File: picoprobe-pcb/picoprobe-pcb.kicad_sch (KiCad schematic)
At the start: 2 parts, among them J1 Conn_01x06_Pin, U1 Pico

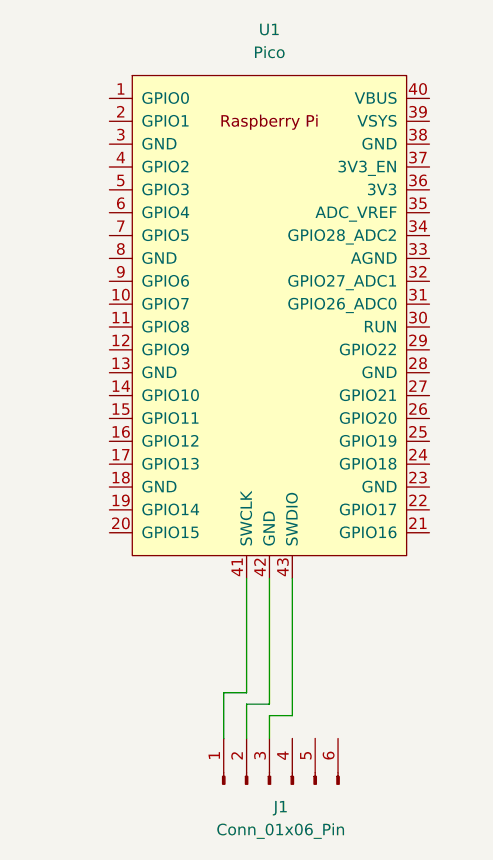
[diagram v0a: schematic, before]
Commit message: First draft
What:

Why:

How:

Tags:
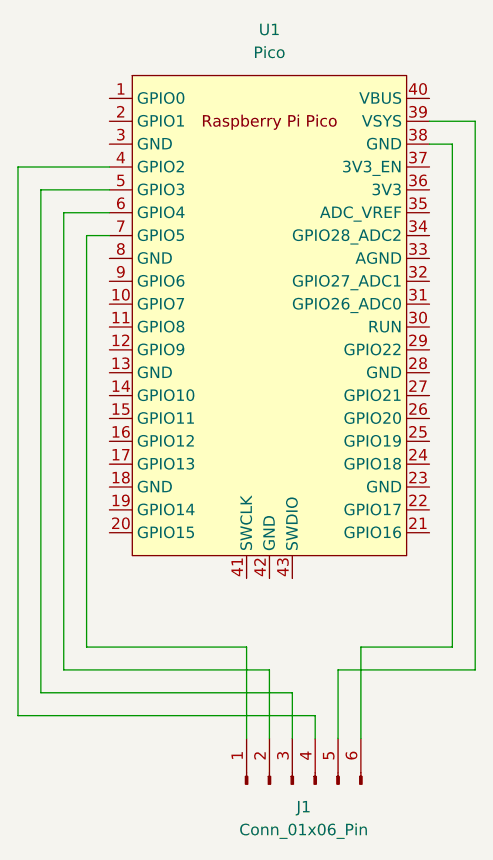
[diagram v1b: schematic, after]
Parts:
- removed U1: Pico, RPi_Pico:RPi_Pico_SMD_TH, symbol RPi_Pico:Pico
- added U1: Pico, MCU_RaspberryPi_and_Boards:RPi_Pico_SMD_TH, symbol MCU_RaspberryPi_and_Boards:Pico
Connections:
- net at J1.1 (Pin_1): now also U1.7 (GPIO5)
- net at J1.2 (Pin_2): now also U1.6 (GPIO4)
- net at J1.3 (Pin_3): now also U1.5 (GPIO3)
- net at J1.4 (Pin_4): now also U1.4 (GPIO2)
- net at J1.5 (Pin_5): now also U1.39 (VSYS)
- net at J1.6 (Pin_6): now also U1.38 (GND)
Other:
- moved on the sheet: J1
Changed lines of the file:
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@@
 (kicad_sch (version 20230121) (generator eeschema)
   (paper "A4")
-  (wire (pts (xy 128.27 127) (xy 128.27 140.97))
+  (wire (pts (xy 110.49 83.82) (xy 102.87 83.82))
     (stroke (width 0) (type default))
   )
-  (wire (pts (xy 128.27 142.24) (xy 128.27 144.78))
+  (wire (pts (xy 110.49 81.28) (xy 100.33 81.28))
     (stroke (width 0) (type default))
   )
-  (wire (pts (xy 130.81 142.24) (xy 128.27 142.24))
+  (wire (pts (xy 105.41 137.16) (xy 128.27 137.16))
     (stroke (width 0) (type default))
   )
-  (wire (pts (xy 128.27 140.97) (xy 125.73 140.97))
+  (wire (pts (xy 135.89 137.16) (xy 135.89 144.78))
     (stroke (width 0) (type default))
   )
-  (wire (pts (xy 130.81 127) (xy 130.81 142.24))
+  (wire (pts (xy 151.13 76.2) (xy 151.13 137.16))
     (stroke (width 0) (type default))
   )
-  (wire (pts (xy 125.73 139.7) (xy 123.19 139.7))
+  (wire (pts (xy 130.81 139.7) (xy 130.81 144.78))
     (stroke (width 0) (type default))
   )
-  (wire (pts (xy 125.73 127) (xy 125.73 139.7))
+  (wire (pts (xy 102.87 139.7) (xy 130.81 139.7))
     (stroke (width 0) (type default))
   )
-  (wire (pts (xy 123.19 139.7) (xy 123.19 144.78))
+  (wire (pts (xy 138.43 134.62) (xy 138.43 144.78))
     (stroke (width 0) (type default))
   )
-  (wire (pts (xy 125.73 140.97) (xy 125.73 144.78))
+  (wire (pts (xy 151.13 76.2) (xy 146.05 76.2))
     (stroke (width 0) (type default))
   )
-  (symbol (lib_id "Connector:Conn_01x06_Pin") (at 128.27 149.86 90) (unit 1)
+  (wire (pts (xy 125.73 134.62) (xy 125.73 144.78))
+    (stroke (width 0) (type default))
+  )
+  (wire (pts (xy 133.35 142.24) (xy 133.35 144.78))
+    (stroke (width 0) (type default))
+  )
+  (wire (pts (xy 151.13 137.16) (xy 135.89 137.16))
+    (stroke (width 0) (type default))
+  )
+  (wire (pts (xy 107.95 134.62) (xy 125.73 134.62))
+    (stroke (width 0) (type default))
+  )
+  (wire (pts (xy 107.95 88.9) (xy 107.95 134.62))
+    (stroke (width 0) (type default))
+  )
+  (wire (pts (xy 110.49 88.9) (xy 107.95 88.9))
+    (stroke (width 0) (type default))
+  )
+  (wire (pts (xy 100.33 142.24) (xy 133.35 142.24))
+    (stroke (width 0) (type default))
+  )
+  (wire (pts (xy 148.59 134.62) (xy 138.43 134.62))
+    (stroke (width 0) (type default))
+  )
+  (wire (pts (xy 105.41 86.36) (xy 105.41 137.16))
+    (stroke (width 0) (type default))
+  )
+  (wire (pts (xy 110.49 86.36) (xy 105.41 86.36))
+    (stroke (width 0) (type default))
+  )
+  (wire (pts (xy 128.27 137.16) (xy 128.27 144.78))
+    (stroke (width 0) (type default))
+  )
+  (wire (pts (xy 102.87 83.82) (xy 102.87 139.7))
+    (stroke (width 0) (type default))
+  )
+  (wire (pts (xy 100.33 81.28) (xy 100.33 142.24))
+    (stroke (width 0) (type default))
+  )
+  (wire (pts (xy 148.59 78.74) (xy 146.05 78.74))
+    (stroke (width 0) (type default))
+  )
+  (wire (pts (xy 148.59 78.74) (xy 148.59 134.62))
+    (stroke (width 0) (type default))
+  )
+  (symbol (lib_id "Connector:Conn_01x06_Pin") (at 130.81 149.86 90) (unit 1)
     (in_bom yes) (on_board yes) (dnp no) (fields_autoplaced)
-    (property "Reference" "J1" (at 129.54 152.4 90)
+    (property "Reference" "J1" (at 132.08 152.4 90)
       (effects (font (size 1.27 1.27)))
     )
-    (property "Value" "Conn_01x06_Pin" (at 129.54 154.94 90)
+    (property "Value" "Conn_01x06_Pin" (at 132.08 154.94 90)
       (effects (font (size 1.27 1.27)))
     )
-    (property "Footprint" "Connector_PinHeader_2.54mm:PinHeader_1x06_P2.54mm_Horizontal" (at 128.27 149.86 0)
+    (property "Footprint" "Connector_PinHeader_2.54mm:PinHeader_1x06_P2.54mm_Horizontal" (at 130.81 149.86 0)
       (effects (font (size 1.27 1.27)) hide)
     )
-    (property "Datasheet" "~" (at 128.27 149.86 0)
+    (property "Datasheet" "~" (at 130.81 149.86 0)
       (effects (font (size 1.27 1.27)) hide)
     )
@@
     )
   )
-  (symbol (lib_id "RPi_Pico:Pico") (at 128.27 97.79 0) (unit 1)
+  (symbol (lib_id "MCU_RaspberryPi_and_Boards:Pico") (at 128.27 97.79 0) (unit 1)
     (in_bom yes) (on_board yes) (dnp no) (fields_autoplaced)
     (property "Reference" "U1" (at 128.27 66.04 0)
@@
       (effects (font (size 1.27 1.27)))
     )
-    (property "Footprint" "RPi_Pico:RPi_Pico_SMD_TH" (at 128.27 97.79 90)
+    (property "Footprint" "MCU_RaspberryPi_and_Boards:RPi_Pico_SMD_TH" (at 128.27 97.79 90)
       (effects (font (size 1.27 1.27)) hide)
     )
